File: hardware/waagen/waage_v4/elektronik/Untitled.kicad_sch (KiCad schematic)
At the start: 9 parts, among them J1 USB_A, J2 Conn_01x03, J3 USB_A, SW1 SW_Push, U1 ATtiny414-SS

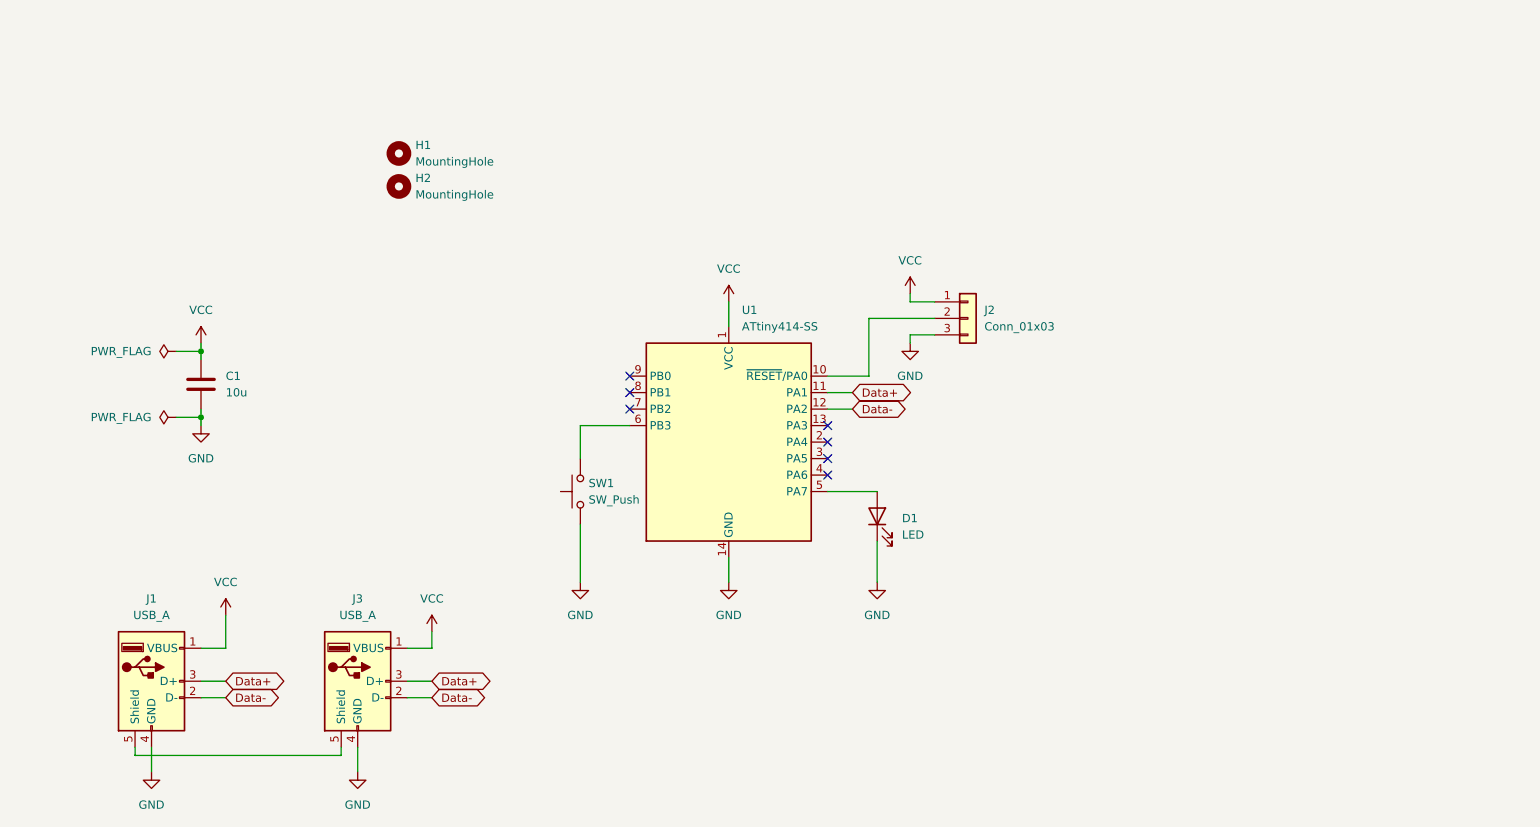
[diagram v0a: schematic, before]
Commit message: intermediate step
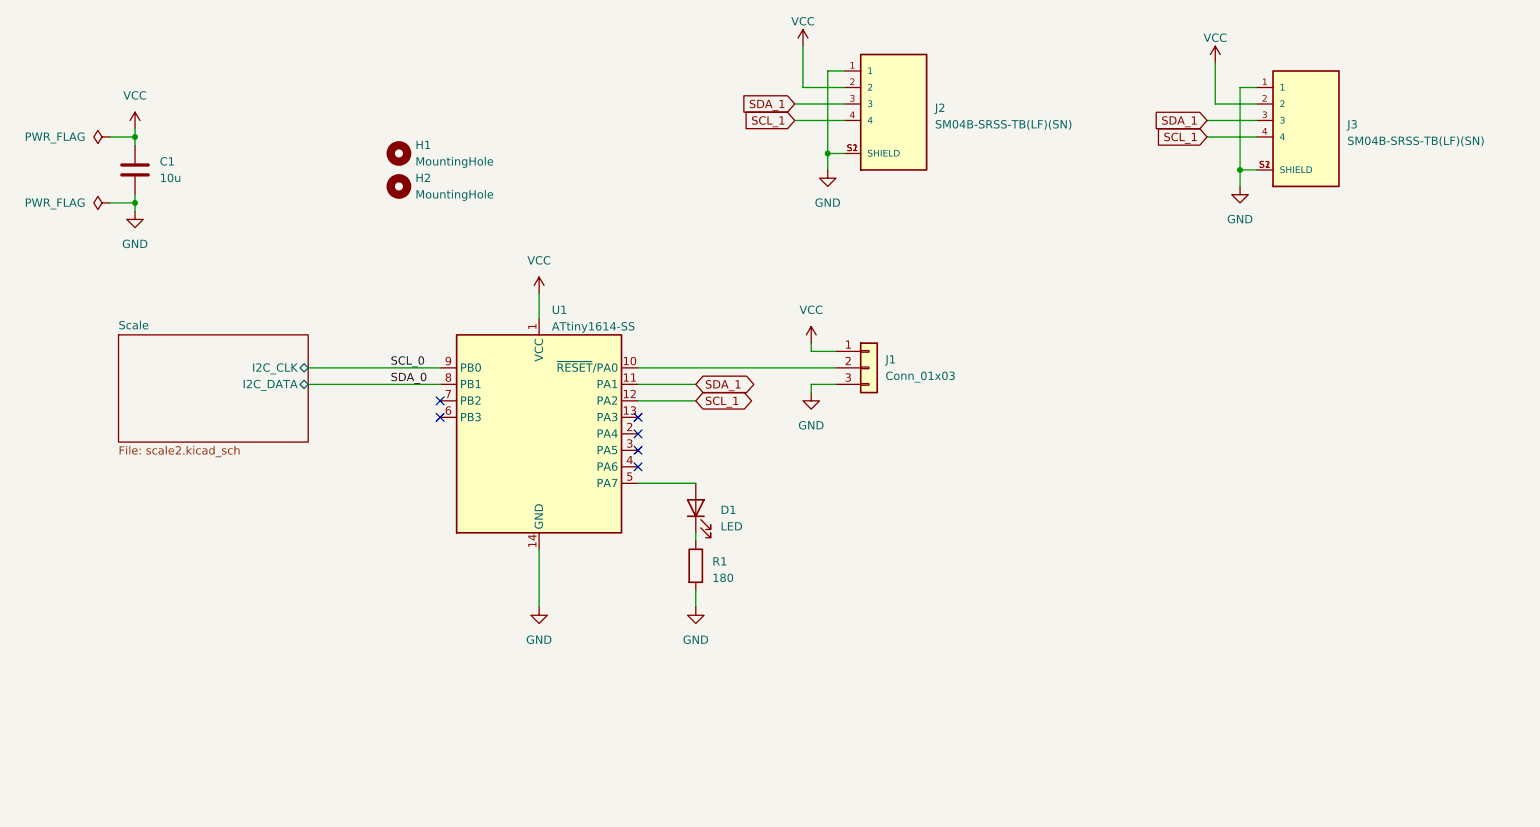
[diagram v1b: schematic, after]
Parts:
- removed J1: USB_A, Library_USB_A:Conn_USB_A_Jack, symbol Connector:USB_A
- removed J3: USB_A, Library_USB_A:Conn_USB_A_Plug, symbol Connector:USB_A
- removed SW1: SW_Push, Library_USB_A:Button_Switch_ESE-11MV1T, symbol Switch:SW_Push
- removed U1: ATtiny414-SS, Package_SO:SOIC-14_3.9x8.7mm_P1.27mm, symbol MCU_Microchip_ATtiny:ATtiny414-SS
- added J2, J3: SM04B-SRSS-TB(LF)(SN), Quiicconnector:JST_SM04B-SRSS-TB(LF)(SN), symbol connector:SM04B-SRSS-TB(LF)(SN)
- added R1: 180, Resistor_SMD:R_1206_3216Metric_Pad1.30x1.75mm_HandSolder, symbol Device:R
- added U1: ATtiny1614-SS, Package_SO:SOIC-14_3.9x8.7mm_P1.27mm, symbol MCU_Microchip_ATtiny:ATtiny1614-SS
- D1: footprint LED_THT:LED_D5.0mm_Horizontal_O3.81mm_Z9.0mm -> LED_SMD:LED_1206_3216Metric_Pad1.42x1.75mm_HandSolder
- renumbered J2 to J1
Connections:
- net GND: now also J2.1, J2.S1 (SHIELD), J2.S2 (SHIELD), J3.1, J3.S1 (SHIELD), J3.S2 (SHIELD), R1.2, U1.14 (GND); no longer D1.1 (K)
- net VCC: now also J2.2, J3.2, U1.1 (VCC)
- net at J1.2 (Pin_2): now also U1.10 (~{RESET}/PA0)
- net at D1.2 (A): now also U1.5 (PA7)
- new net: D1.1 (K), R1.1
- new net SCL_0: U1.9 (PB0)
- new net SCL_1: J2.4, J3.4, U1.12 (PA2)
- new net SDA_0: U1.8 (PB1)
- new net SDA_1: J2.3, J3.3, U1.11 (PA1)
- no-connect marks 7 -> 6
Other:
- added sheet Scale (scale2.kicad_sch)
- moved on the sheet: C1, D1, J1
